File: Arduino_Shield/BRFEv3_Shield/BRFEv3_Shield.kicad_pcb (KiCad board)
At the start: 2 copper layers, 68.6 x 53.3 mm, 8 parts, among them P1 Power, P2 Analog, P3 Digital, P4 Digital, P5 CONN_01X01, P6 CONN_01X01, P7 CONN_01X01, P8 CONN_01X01

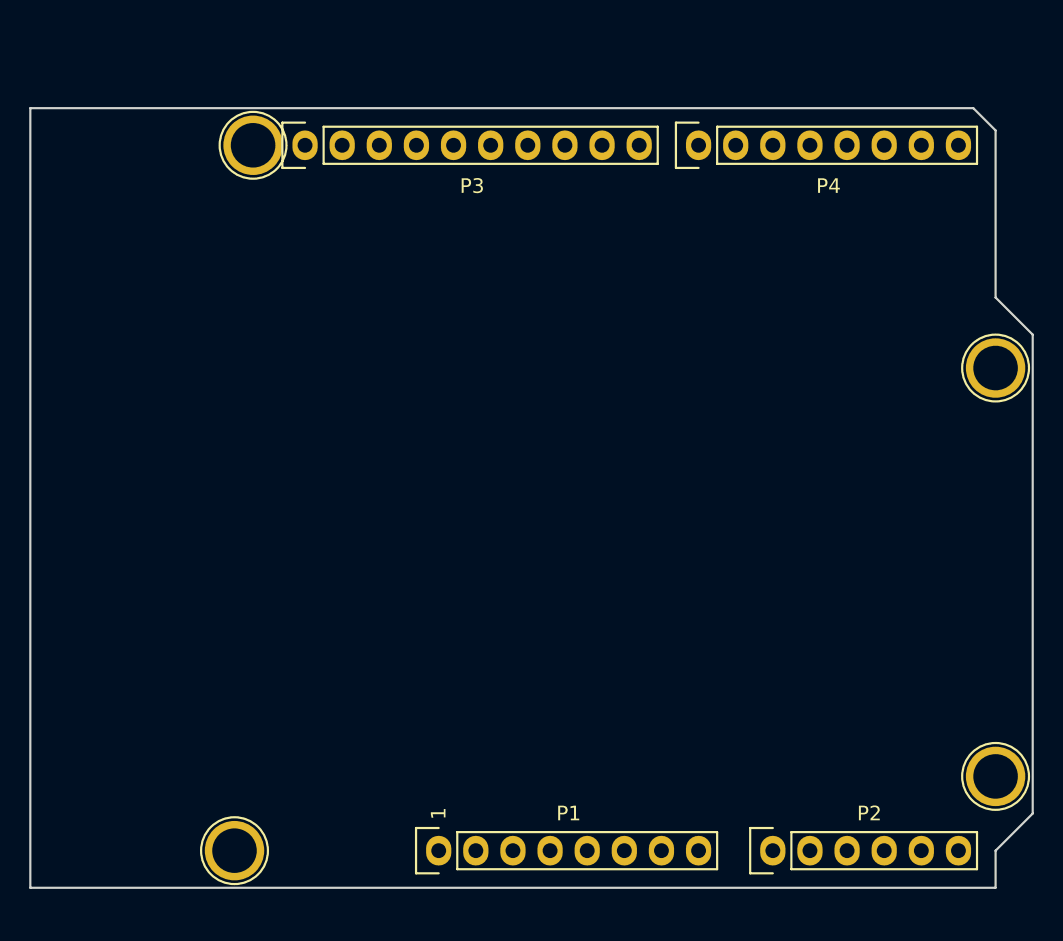
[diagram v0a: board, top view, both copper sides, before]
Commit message: update shield
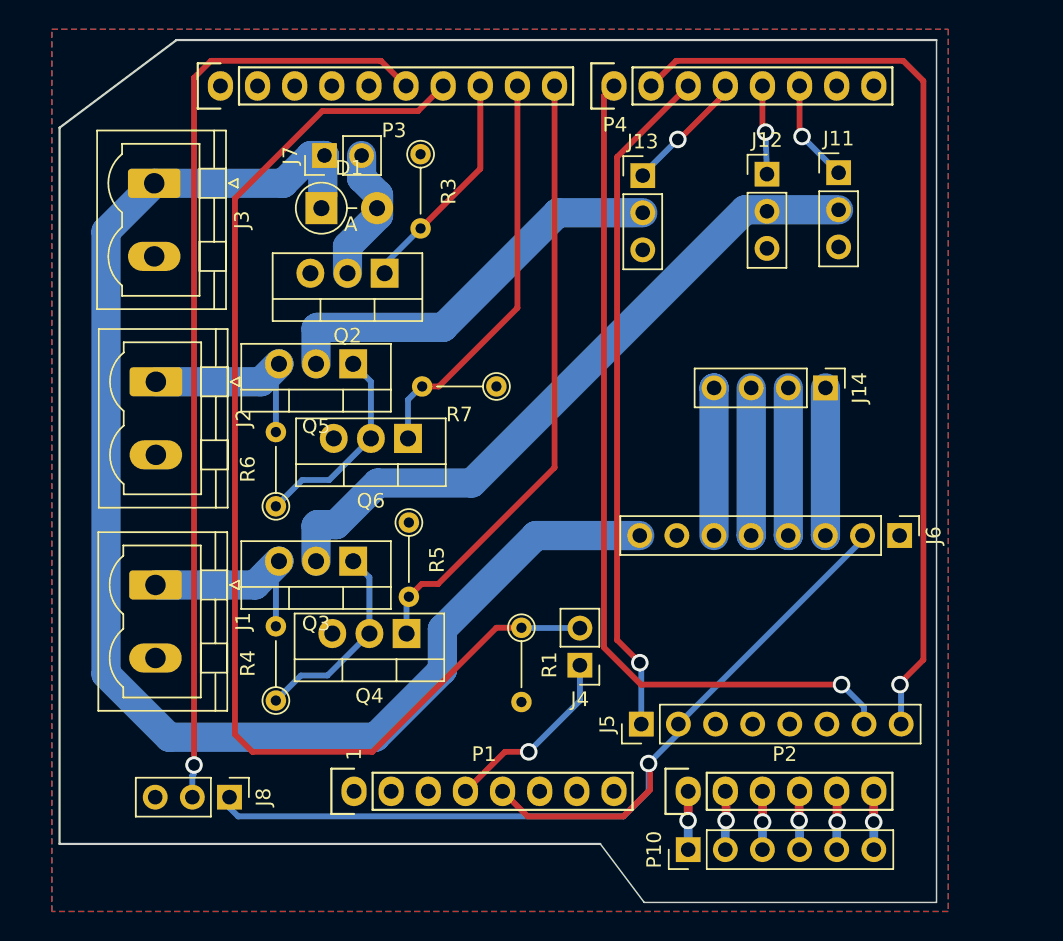
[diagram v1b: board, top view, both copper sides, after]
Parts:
- removed P5, P6, P7, P8: CONN_01X01, Socket_Arduino_Uno:Arduino_1pin
- added D1: D, Diode_THT:D_DO-41_SOD81_P3.81mm_Vertical_AnodeUp, F.Cu at (130.9, 79.9)
- added J1: Screw_Terminal_01x02, Connector_Phoenix_MSTB:PhoenixContact_MSTBVA_2,5_2-G_1x02_P5.00mm_Vertical, F.Cu at (119.6, 105.6)
- added J11: Servo1, Connector_PinHeader_2.54mm:PinHeader_1x03_P2.54mm_Vertical, F.Cu at (166.3, 77.4)
- added J12: Servo2, Connector_PinHeader_2.54mm:PinHeader_1x03_P2.54mm_Vertical, F.Cu at (161.4, 77.5)
- added J13: Pince, Connector_PinHeader_2.54mm:PinHeader_1x03_P2.54mm_Vertical, F.Cu at (152.9, 77.6)
- added J14: Pas-à-pas, Connector_PinHeader_2.54mm:PinHeader_1x04_P2.54mm_Vertical, F.Cu at (165.4, 92.2)
- added J2: Screw_Terminal_01x02, Connector_Phoenix_MSTB:PhoenixContact_MSTBVA_2,5_2-G_1x02_P5.00mm_Vertical, F.Cu at (119.6, 91.7)
- added J3: Screw_Terminal_01x02, Connector_Phoenix_MSTB:PhoenixContact_MSTBVA_2,5_2-G_1x02_P5.00mm_Vertical, F.Cu at (119.5, 78.2)
- added J4: FDC, Connector_PinHeader_2.54mm:PinHeader_1x02_P2.54mm_Vertical, F.Cu at (148.6, 111.1)
- added J5: Conn_01x08_Female, Connector_PinHeader_2.54mm:PinHeader_1x08_P2.54mm_Vertical, F.Cu at (152.8, 115.2)
- added J6: Conn_01x08_Female, Connector_PinHeader_2.54mm:PinHeader_1x08_P2.54mm_Vertical, F.Cu at (170.5, 102.3)
- added J7: FAN, Connector_PinHeader_2.54mm:PinHeader_1x02_P2.54mm_Vertical, F.Cu at (131.1, 76.3)
- added J8: DHT22, Connector_PinHeader_2.54mm:PinHeader_1x03_P2.54mm_Vertical, F.Cu at (124.6, 120.2)
- added P10: Analog, Connector_PinHeader_2.54mm:PinHeader_1x06_P2.54mm_Vertical, F.Cu at (156.0, 123.8)
- added Q2: IRL510PBF, Package_TO_SOT_THT:TO-220-3_Vertical, F.Cu at (135.2, 84.3)
- added Q3: IRF4905, Package_TO_SOT_THT:TO-220-3_Vertical, F.Cu at (133.1, 104.0)
- added Q4: IRL510PBF, Package_TO_SOT_THT:TO-220-3_Vertical, F.Cu at (136.7, 109.0)
- added Q5: IRF4905, Package_TO_SOT_THT:TO-220-3_Vertical, F.Cu at (133.1, 90.5)
- added Q6: IRL510PBF, Package_TO_SOT_THT:TO-220-3_Vertical, F.Cu at (136.8, 95.6)
- added R1: 10k, Resistor_THT:R_Axial_DIN0204_L3.6mm_D1.6mm_P5.08mm_Vertical, F.Cu at (144.6, 108.6)
- added R3: 10k, Resistor_THT:R_Axial_DIN0204_L3.6mm_D1.6mm_P5.08mm_Vertical, F.Cu at (137.7, 76.2)
- added R4: 10k, Resistor_THT:R_Axial_DIN0204_L3.6mm_D1.6mm_P5.08mm_Vertical, F.Cu at (127.8, 113.6)
- added R5: 10k, Resistor_THT:R_Axial_DIN0204_L3.6mm_D1.6mm_P5.08mm_Vertical, F.Cu at (136.9, 101.4)
- added R6: 10k, Resistor_THT:R_Axial_DIN0204_L3.6mm_D1.6mm_P5.08mm_Vertical, F.Cu at (127.8, 100.3)
- added R7: 10k, Resistor_THT:R_Axial_DIN0204_L3.6mm_D1.6mm_P5.08mm_Vertical, F.Cu at (142.9, 92.1)
- moved P3 7.07 mm to (124.0, 71.5)
- moved P1 7.07 mm to (133.1, 119.8)
- moved P2 7.07 mm to (156.0, 119.8)
- moved P4 7.07 mm to (150.9, 71.5)
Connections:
- P1 pad 1: Net-(P1-Pad1) -> unconnected-(P1-Pad1)
- P3 pad 7: /11(**/MOSI) -> /11(**/MOSI)
- P3 pad 8: /10(**/SS) -> /10(**/SS)
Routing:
- net +12V: track 0.00 -> 95.8 mm
- net +5V: track 0.00 -> 82.2 mm, vias 0 -> 1
- net /11(**/MOSI): track 0.00 -> 81.7 mm
- net /6(**): track 0.00 -> 64.7 mm, vias 0 -> 1
- net /12(MISO): track 0.00 -> 64.4 mm, vias 0 -> 1
- net /7: track 0.00 -> 59.3 mm, vias 0 -> 1
- net /big_servo_control: track 0.00 -> 47.1 mm
- net /5(**): track 0.00 -> 46.4 mm, vias 0 -> 1
- net /8: track 0.00 -> 42.2 mm
- net /pince_control: track 0.00 -> 28.0 mm
- net /9(**): track 0.00 -> 27.9 mm
- net /10(**/SS): track 0.00 -> 15.5 mm
- net +6V: track 0.00 -> 14.9 mm
- net Net-(Q5-Pad1): track 0.00 -> 14.0 mm
- net Net-(Q3-Pad1): track 0.00 -> 13.7 mm
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- added copper zone on B.Cu, net GND
- added copper zone on F.Cu, net GND
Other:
- board size 68.6 x 53.3 mm -> 60 x 59 mm
- board text added: "12V"
- board text added: "5V"
- board text added: "6V"
- board text added: "FAN"
- board text added: "FDC"
- board text added: "Pince"
- board text added: "Servo1"
- board text added: "Servo2"
- board text added: "Temp."
- board text added: "Translation"
